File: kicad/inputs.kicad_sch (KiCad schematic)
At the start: 15 parts, among them J5 Thonkiconn, Q1 S8050, U5 MCP6002-xSN, U6 ADC121C027CIMK

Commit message: reroute pcb
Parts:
- J5: footprint Eurorack:Thonkiconn Mono Jack -> allen-synthesis:jack-thonkiconn-mono
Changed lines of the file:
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@@
       (effects (font (size 1.27 1.27)) (justify right))
     )
-    (property "Footprint" "Eurorack:Thonkiconn Mono Jack" (at 41.91 111.76 0)
+    (property "Footprint" "allen-synthesis:jack-thonkiconn-mono" (at 41.91 111.76 0)
       (effects (font (size 1.27 1.27)) hide)
     )
@@
       (effects (font (size 1.27 1.27)) (justify right))
     )
-    (property "Footprint" "Eurorack:Thonkiconn Mono Jack" (at 41.91 60.96 0)
-      (effects (font (size 1.27 1.27)) hide)
-    )
+    (property "Footprint" "allen-synthesis:jack-thonkiconn-mono" (at 41.91 60.96 0)
+      (effects (font (size 1.27 1.27)) hide)
+    )

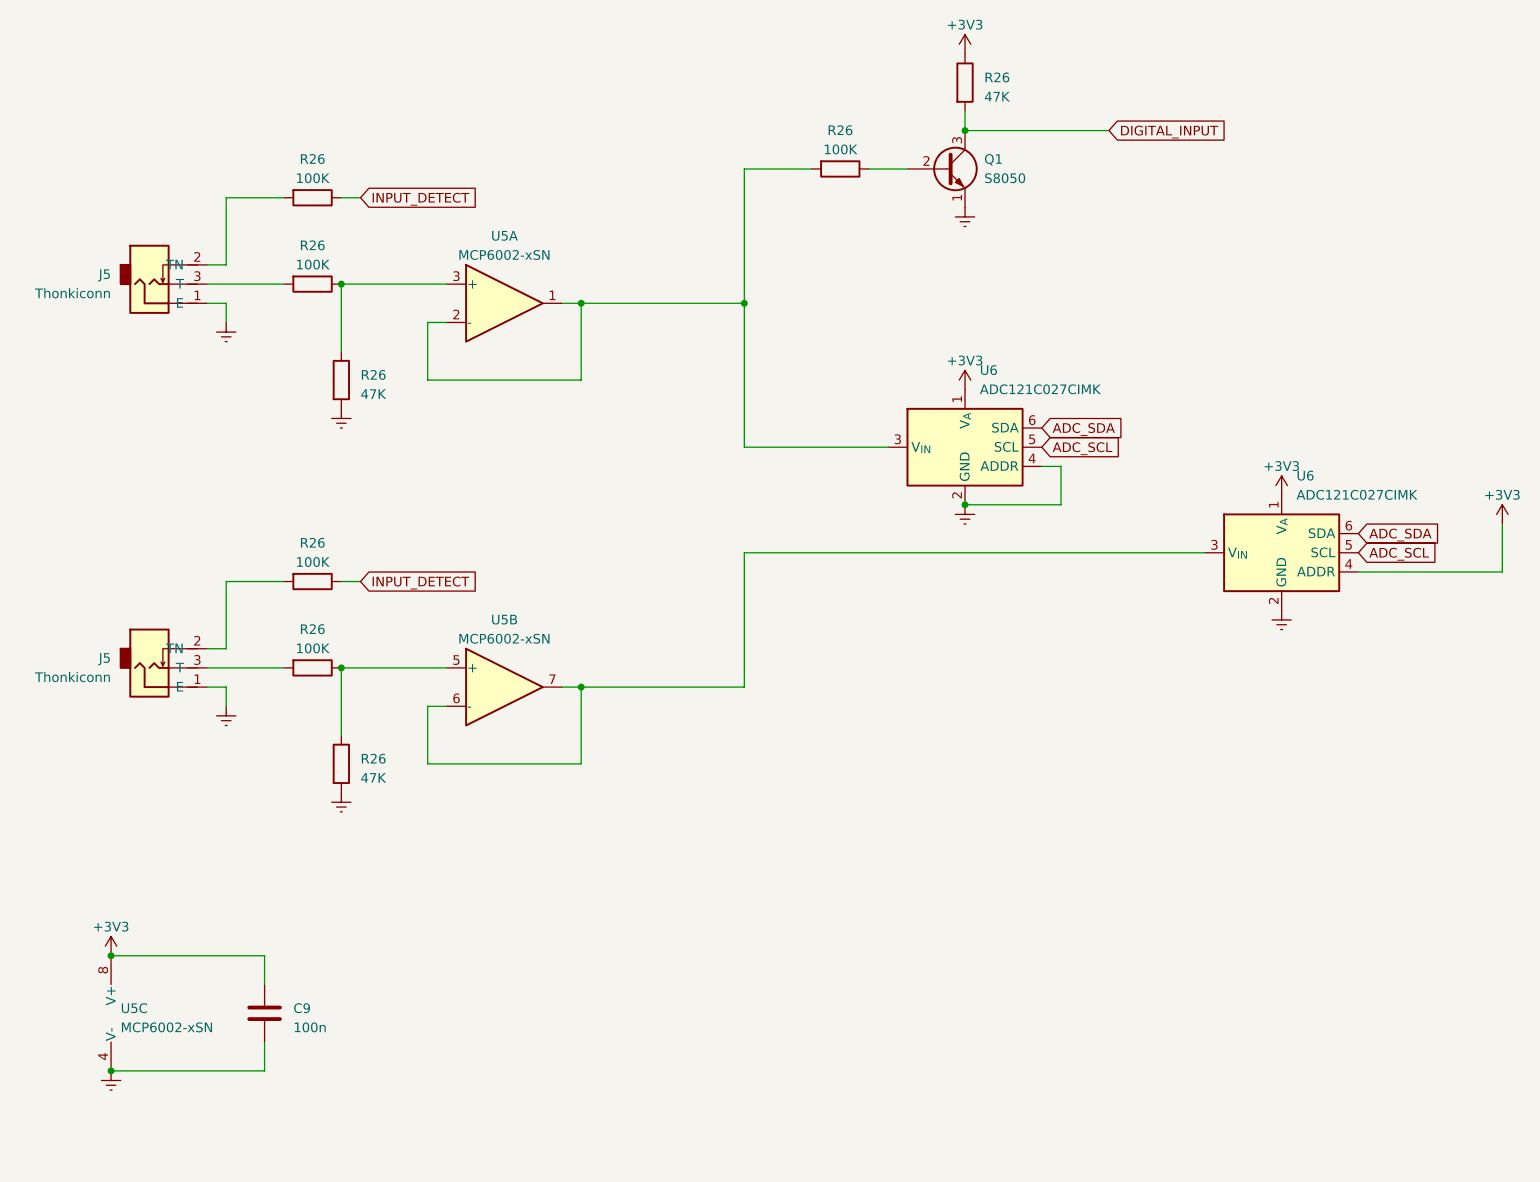
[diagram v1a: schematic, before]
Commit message: add schematic notes
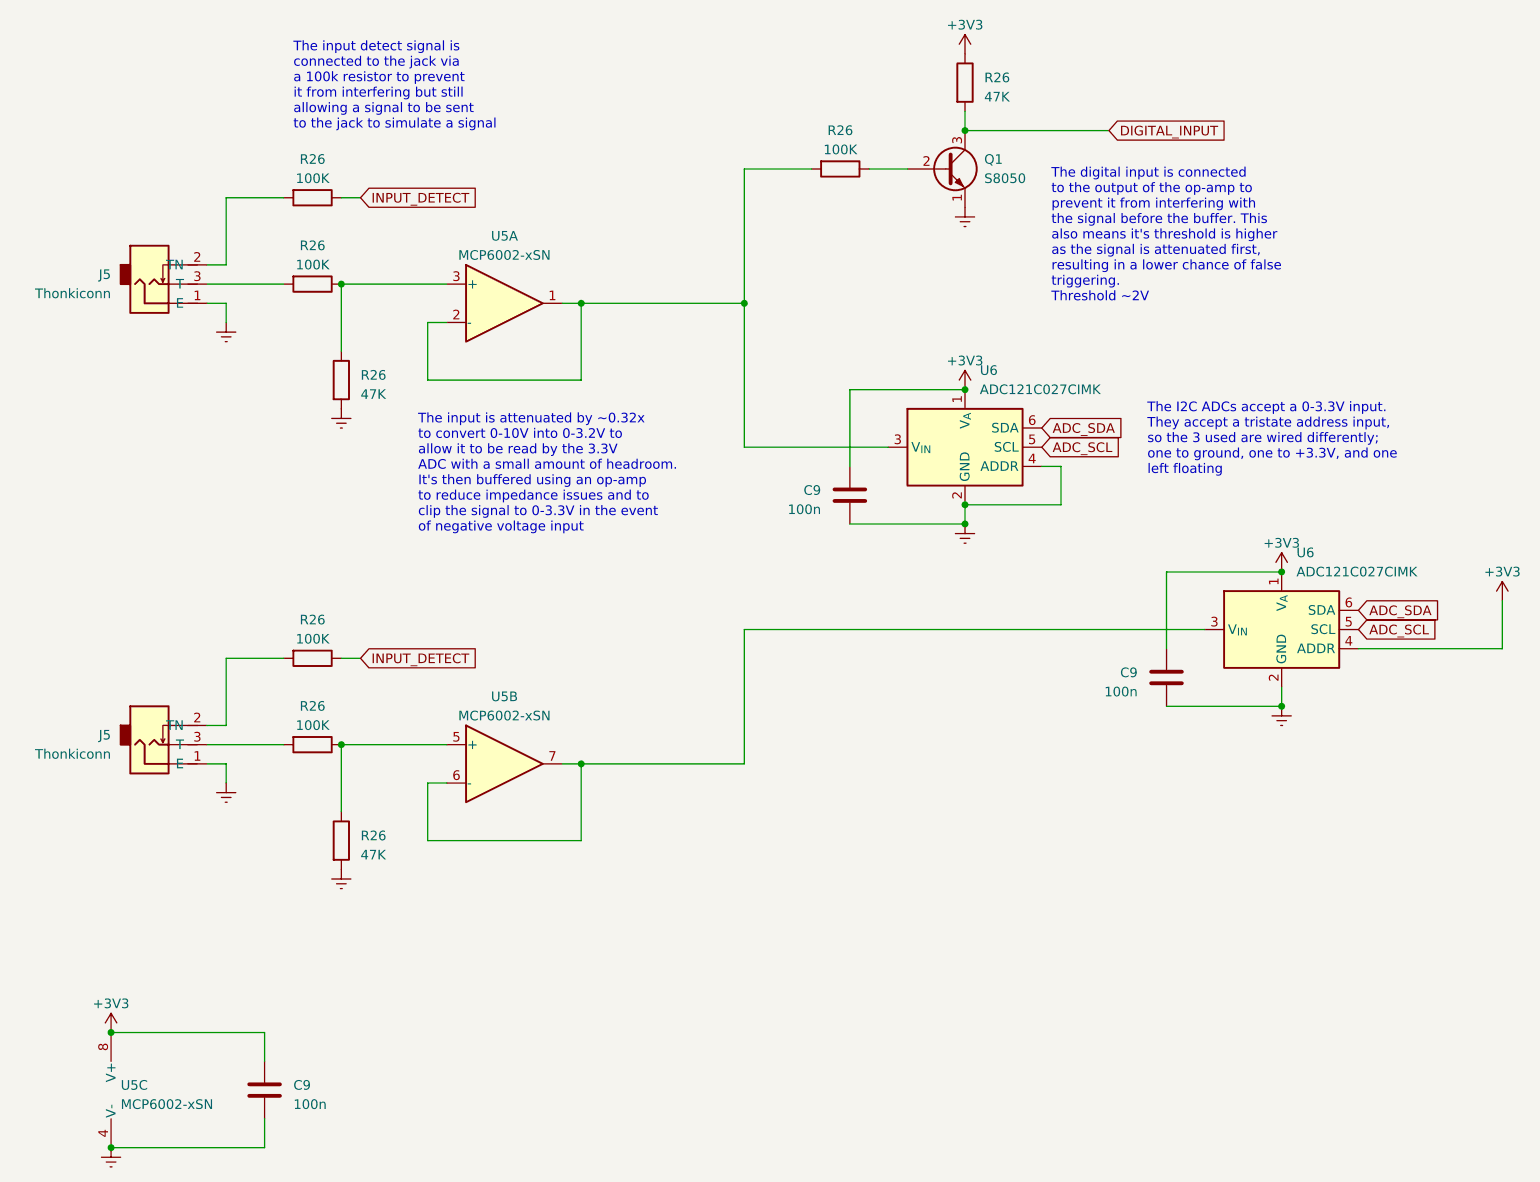
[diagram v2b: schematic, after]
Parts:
- added C9 (x2): 100n, Capacitor_SMD:C_0402_1005Metric, symbol Device:C
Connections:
- net +3V3: now also C9.1, C9.1
- net Earth: now also C9.2, C9.2
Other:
- note added: "The I2C ADCs accept a 0-3.3V input. They accept a tristate address input, so the 3 used are wired differently; one to ground, one to +3.3V, and one left floating"
- note added: "The digital input is connected to the output of the op-amp to prevent it from interfering with the signal before the buffer. This also means it's threshold is higher as the signal is attenuated first, resulting in a lower chance of false triggering. Threshold ~2V"
- note added: "The input detect signal is connected to the jack via a 100k resistor to prevent it from interfering but still allowing a signal to be sent to the jack to simulate a signal"
- note added: "The input is attenuated by ~0.32x to convert 0-10V into 0-3.2V to allow it to be read by the 3.3V ADC with a small amount of headroom. It's then buffered using an op-amp to reduce impedance issues and to clip the signal to 0-3.3V in the event of negative voltage input"
- moved on the sheet: C9, J5, R26, U5B, U5C, U6
